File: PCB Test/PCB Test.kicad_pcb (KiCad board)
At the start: 2 copper layers, 164 x 99 mm, 47 parts, among them J1 Motor Terminal 2, J2 Conn_02x05_Odd_Even, J5 Motor Terminal 1, J6 Conn_02x03_Odd_Even, Q2 NMOS, Q3 NMOS, SW1 SW_Push, SW2 SW_Push, SW3 SW_Push, U1 ATmega4808-A, U2 TCRT5000, U3 TCRT5000, U4 TCRT5000, U5 MCP1700x-330xxTO

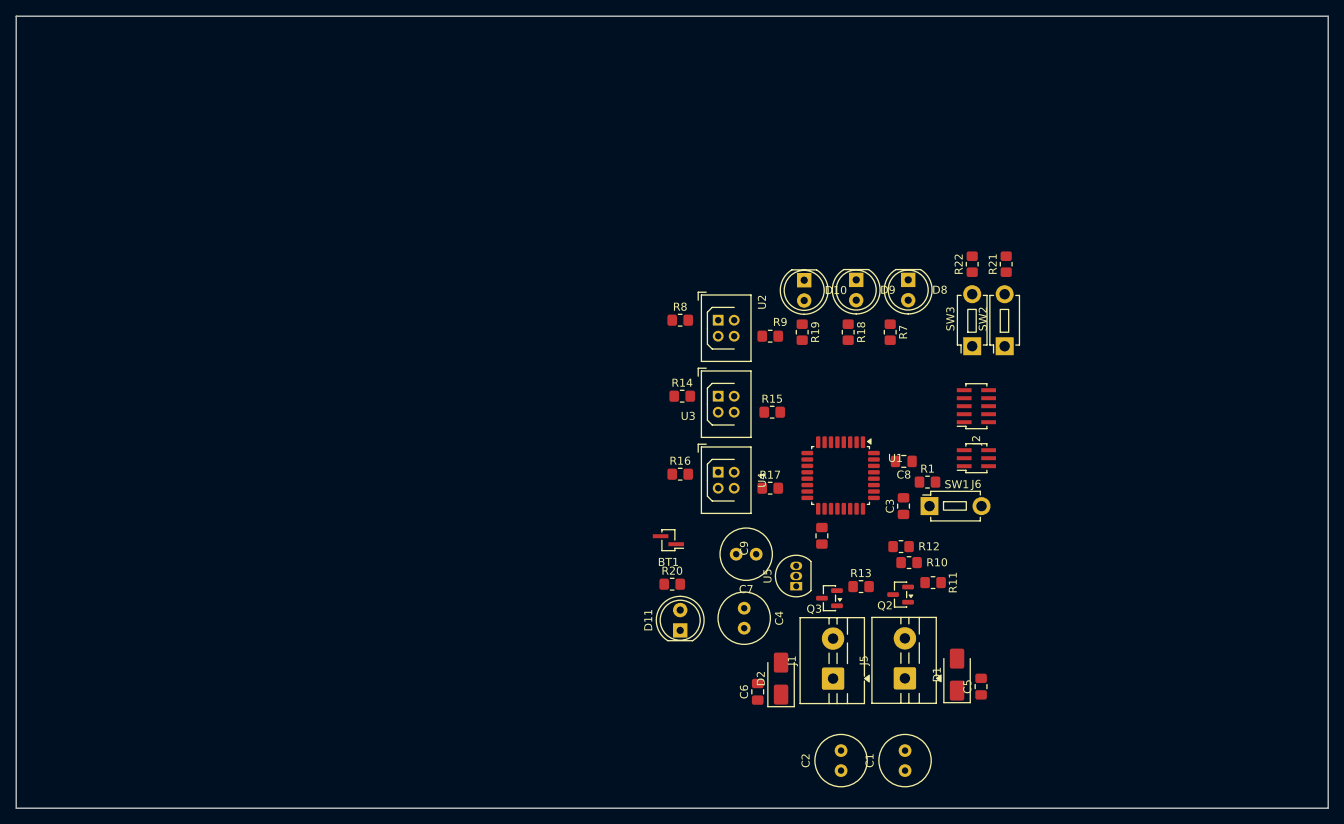
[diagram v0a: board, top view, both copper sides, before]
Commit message: Final layout finished, moving on to motion transmition, need to extract gerber files
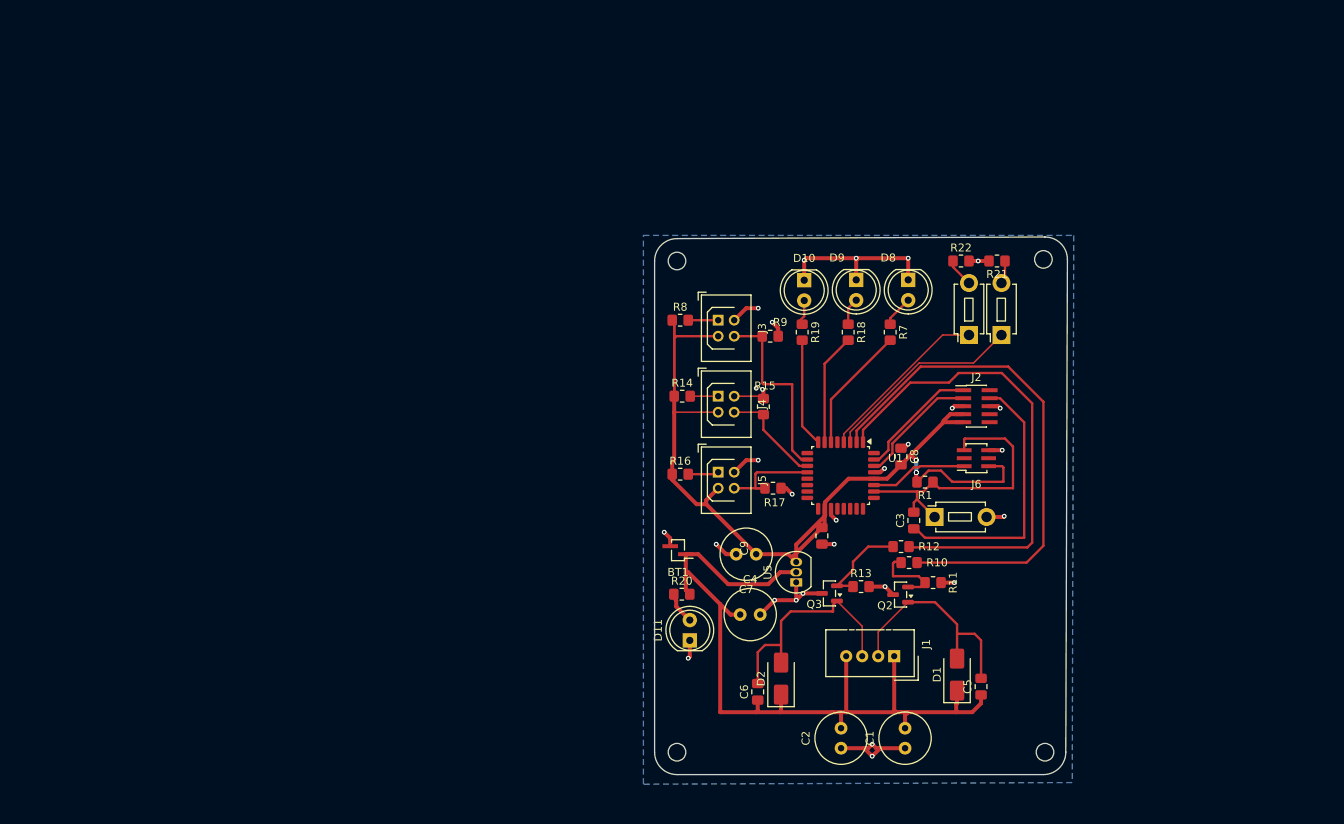
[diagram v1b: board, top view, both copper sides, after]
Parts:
- removed U2, U3, U4: TCRT5000, Connector_Harwin:Harwin_LTek-Male_2x02_P2.00mm_Vertical
- added H1: MountingHole, MountingHole:MountingHole_2.2mm_M2, F.Cu at (135.6, 91.6)
- added H2: MountingHole, MountingHole:MountingHole_2.2mm_M2, F.Cu at (181.4, 91.4)
- added H3: MountingHole, MountingHole:MountingHole_2.2mm_M2, F.Cu at (181.6, 153.0)
- added H4: MountingHole, MountingHole:MountingHole_2.2mm_M2, F.Cu at (135.6, 153.0)
- added J3: Conn_02x02_Odd_Even, Connector_Harwin:Harwin_LTek-Male_2x02_P2.00mm_Vertical, F.Cu at (140.8, 99.0)
- added J4: Conn_02x02_Odd_Even, Connector_Harwin:Harwin_LTek-Male_2x02_P2.00mm_Vertical, F.Cu at (140.8, 108.5)
- J1: value Motor Terminal 2 -> Conn_02x02_Counter_Clockwise; footprint TerminalBlock:TerminalBlock_MaiXu_MX126-5.0-02P_1x02_P5.00mm -> Connector:NS-Tech_Grove_1x04_P2mm_Vertical
- J2: footprint Connector_PinSocket_1.00mm:PinSocket_2x05_P1.00mm_Vertical_SMD -> Connector_PinHeader_1.00mm:PinHeader_2x05_P1.00mm_Vertical_SMD
- J5: value Motor Terminal 1 -> Conn_02x02_Odd_Even; footprint TerminalBlock:TerminalBlock_MaiXu_MX126-5.0-02P_1x02_P5.00mm -> Connector_Harwin:Harwin_LTek-Male_2x02_P2.00mm_Vertical
- moved J5 34.8 mm to (140.8, 118.0), turned to -90 degrees
- moved J1 8.14 mm to (162.8, 141.0), turned to -90 degrees
- moved C1 2.80 mm to (164.1, 152.5)
- moved C2 2.80 mm to (156.1, 152.5)
- moved C3 2.21 mm to (165.2, 124.0)
- moved BT1 1.73 mm to (135.7, 127.8)
- moved D11 1.73 mm to (137.2, 139.0)
- moved R20 1.73 mm to (136.2, 133.2)
- moved SW1 1.50 mm to (167.8, 123.6)
- moved R22 1.46 mm to (171.1, 91.6), turned to 0 degrees
- moved SW3 1.46 mm to (172.1, 100.8)
- moved SW2 1.46 mm to (176.2, 100.9)
- moved R15 1.30 mm to (146.4, 109.8), turned to 90 degrees
- moved R21 1.22 mm to (175.6, 91.6), turned to 180 degrees
- moved C4 0.94 mm to (143.5, 135.8), turned to 0 degrees
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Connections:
- net USART_RX renamed USART RX
- net USART_TX renamed USART TX
- J1 pad 2: Net-(D2-A) -> Net-(D1-A)
- J5 pad 1: +4.8V -> Net-(J5-Pin_1)
- J5 pad 2: Net-(D1-A) -> +3.3V
- R10 pad 1: Motor 1 -> Motor 2
- R12 pad 1: Motor 2 -> Motor 1
- R16 pad 2: Net-(R16-Pad2) -> Net-(J5-Pin_1)
- R17 pad 1: ADC Sensor 3 -> ADC Sensor 1
- R9 pad 1: ADC Sensor 1 -> ADC Sensor 3
- U1 pad 6: LED_Red -> LED Red
- U1 pad 7: LED Green -> LED Green 1
- U1 pad 8: LED Blue -> LED Green 2
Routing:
- net +3.3V: track 0.00 -> 124.7 mm, vias 0 -> 5
- net +4.8V: track 0.00 -> 102.7 mm
- net GND: track 0.00 -> 87.4 mm, vias 0 -> 27
- net Motor 2: track 0.00 -> 64.6 mm
- net Motor 1: track 0.00 -> 60.3 mm
- net RESET: track 0.00 -> 36.8 mm
- net DTR: track 0.00 -> 34.3 mm
- net Net-(D2-A): track 0.00 -> 29.1 mm
- net Net-(D1-A): track 0.00 -> 27.9 mm
- net Button 1: track 0.00 -> 25.2 mm
- net ADC Sensor 3: track 0.00 -> 23.8 mm
- net Button 2: track 0.00 -> 21.8 mm
- net LED Red: track 0.00 -> 15.8 mm
- net USART TX: track 0.00 -> 15.4 mm
- net USART RX: track 0.00 -> 15.4 mm
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- added copper zone on B.Cu, net GND
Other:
- board size 164 x 99 mm -> 51.6 x 67.2 mm
